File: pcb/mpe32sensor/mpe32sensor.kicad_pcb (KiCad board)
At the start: 2 copper layers, 16 x 21 mm, 9 parts, among them J1 Conn_01x04, J2 Conn_01x01, J3 Conn_01x01, U1 TMAG5273

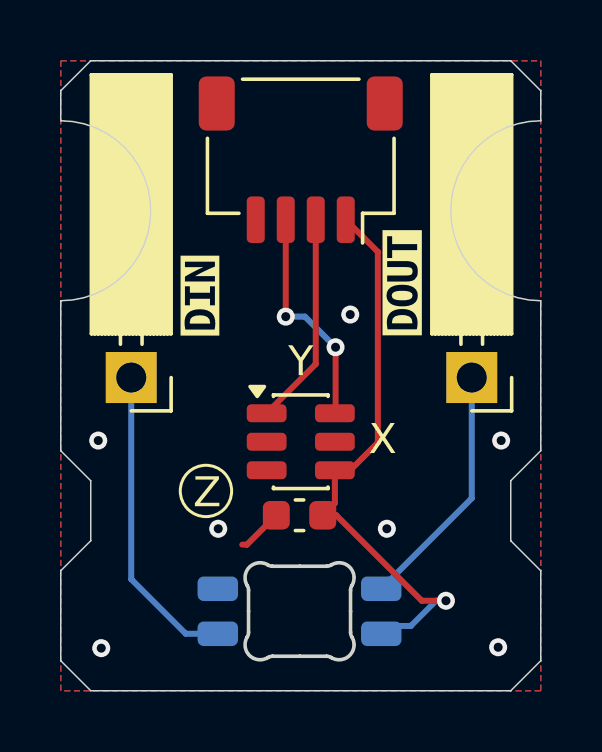
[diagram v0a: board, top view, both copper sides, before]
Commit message: production file changes + ide setup
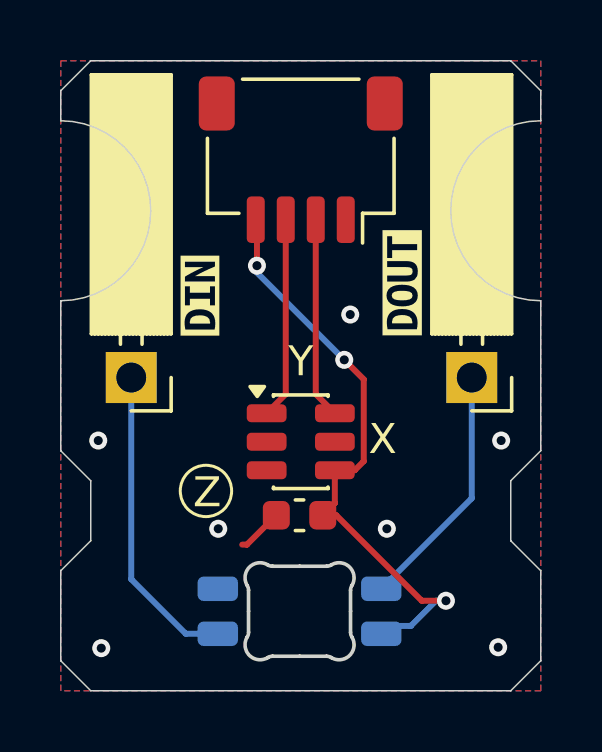
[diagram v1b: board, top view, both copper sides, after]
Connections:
- J1 pad 1: +3V3 -> GND
- J1 pad 2: TMAG5273_SCL -> TMAG5273_SDA
- J1 pad 3: TMAG5273_SDA -> TMAG5273_SCL
- J1 pad 4: GND -> +3V3
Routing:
- net +3V3: track 19.2 -> 20.2 mm, vias 1 -> 3
- net TMAG5273_SDA: track 7.52 -> 6.75 mm, vias 2 -> 0
